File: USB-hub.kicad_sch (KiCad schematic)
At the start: 11 parts, among them U900 CH334R, Y900 12Mhz

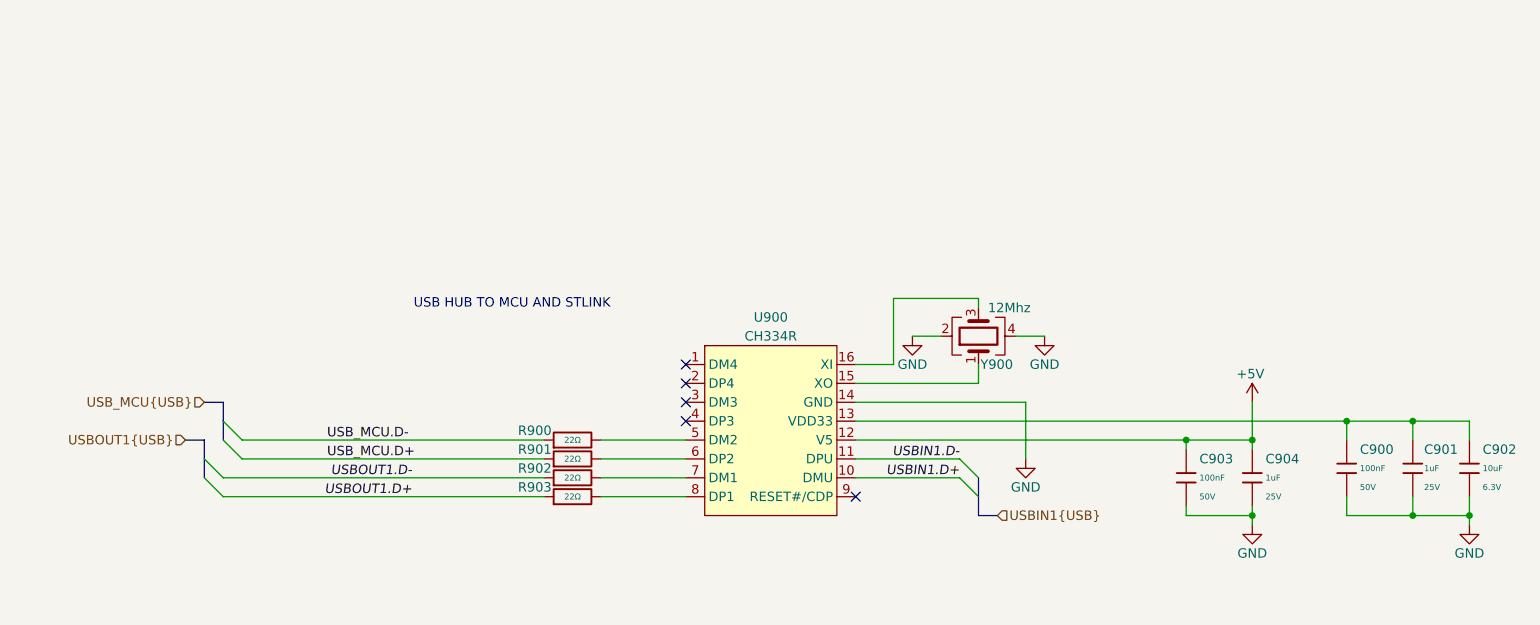
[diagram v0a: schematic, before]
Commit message: Change CH334R to CH334P
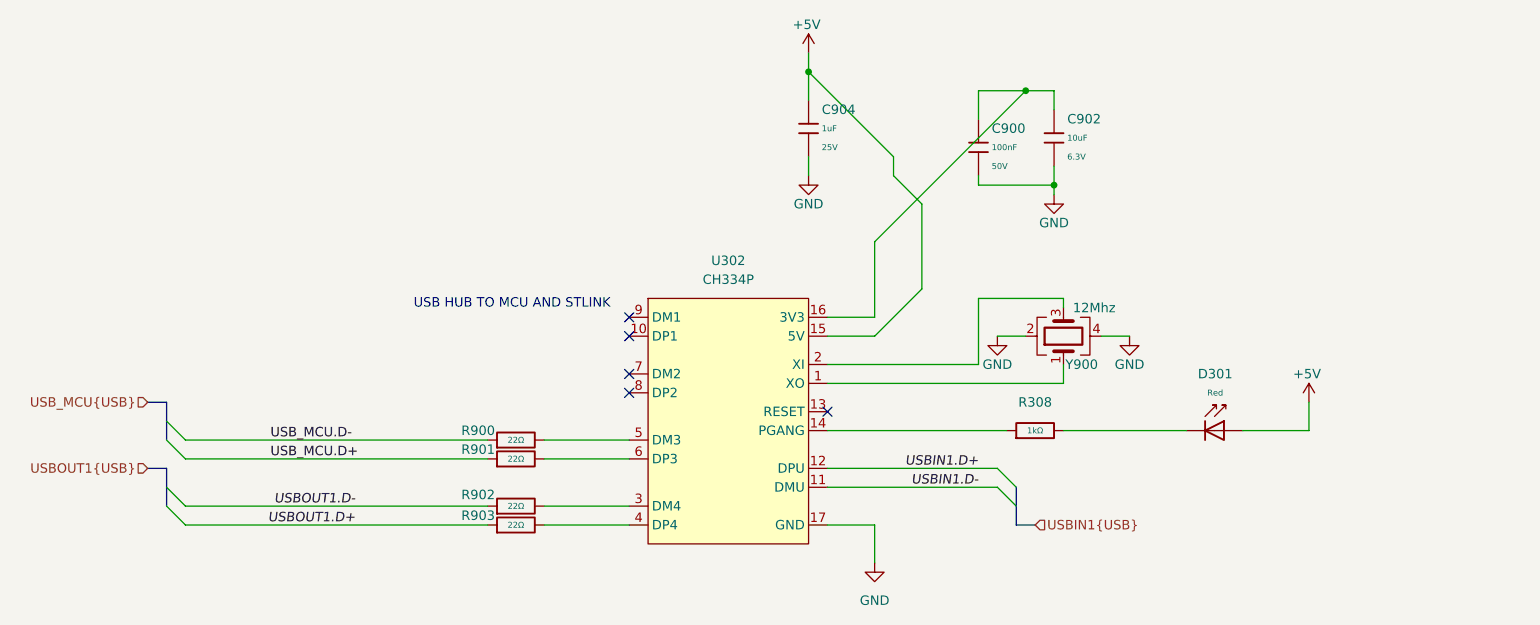
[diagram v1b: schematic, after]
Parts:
- removed C901: 1uF, PCM_JLCPCB:C_0402, symbol PCM_JLCPCB-Capacitors:0402,1uF
- removed C903: 100nF, PCM_JLCPCB:C_0402, symbol PCM_JLCPCB-Capacitors:0402,100nF,(2)
- removed U900: CH334R, Package_SO:QSOP-16_3.9x4.9mm_P0.635mm, symbol WCH_USB:CH334R
- added D301: Red, PCM_JLCPCB:D_0603, symbol PCM_JLCPCB-Diodes:LED,0603,Red
- added R308: 1kΩ, PCM_JLCPCB:R_0402, symbol PCM_JLCPCB-Resistors:0402,1kΩ
- added U302: CH334P, Package_DFN_QFN:QFN-16-1EP_3x3mm_P0.5mm_EP1.7x1.7mm, symbol CH334P:CH334P
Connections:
- net +5V: now also D301.2, U302.15 (5V)
- net GND: now also U302.17 (GND)
- net USBIN1.D+: now also U302.12 (DPU)
- net USBIN1.D-: now also U302.11 (DMU)
- net at R900.2: now also U302.5 (DM3)
- net at C900.1, C902.1: now also U302.16 (3V3)
- net at R902.2: now also U302.3 (DM4)
- net at R903.2: now also U302.4 (DP4)
- net at R901.2: now also U302.6 (DP3)
- net at Y900.1: now also U302.1 (XO)
- net at Y900.3: now also U302.2 (XI)
- new net: R308.1, U302.14 (PGANG)
- new net: D301.1, R308.2
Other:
- moved on the sheet: C900, C902, C904, R900, R901, R902, R903, Y900
